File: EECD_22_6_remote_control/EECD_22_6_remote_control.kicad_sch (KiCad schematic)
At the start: 22 parts, among them SW1 SW_SPDT, U1 NRF24L01_Breakout, U2 NUCLEO144-F746ZG

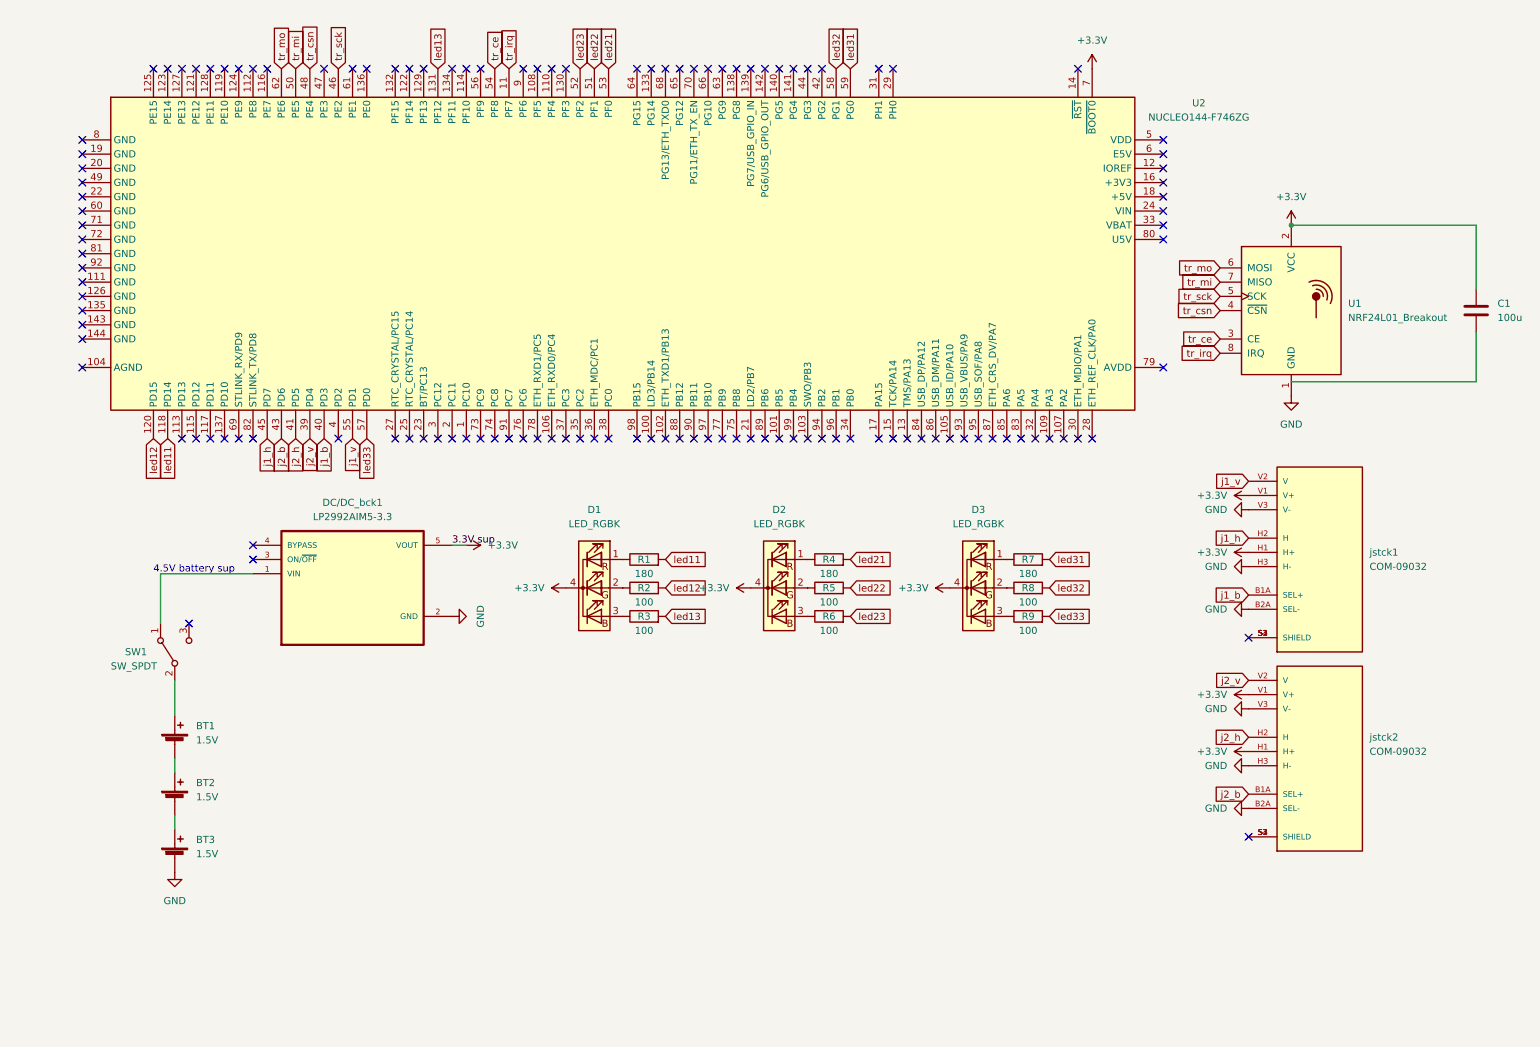
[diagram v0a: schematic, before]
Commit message: you can understand at least smth now
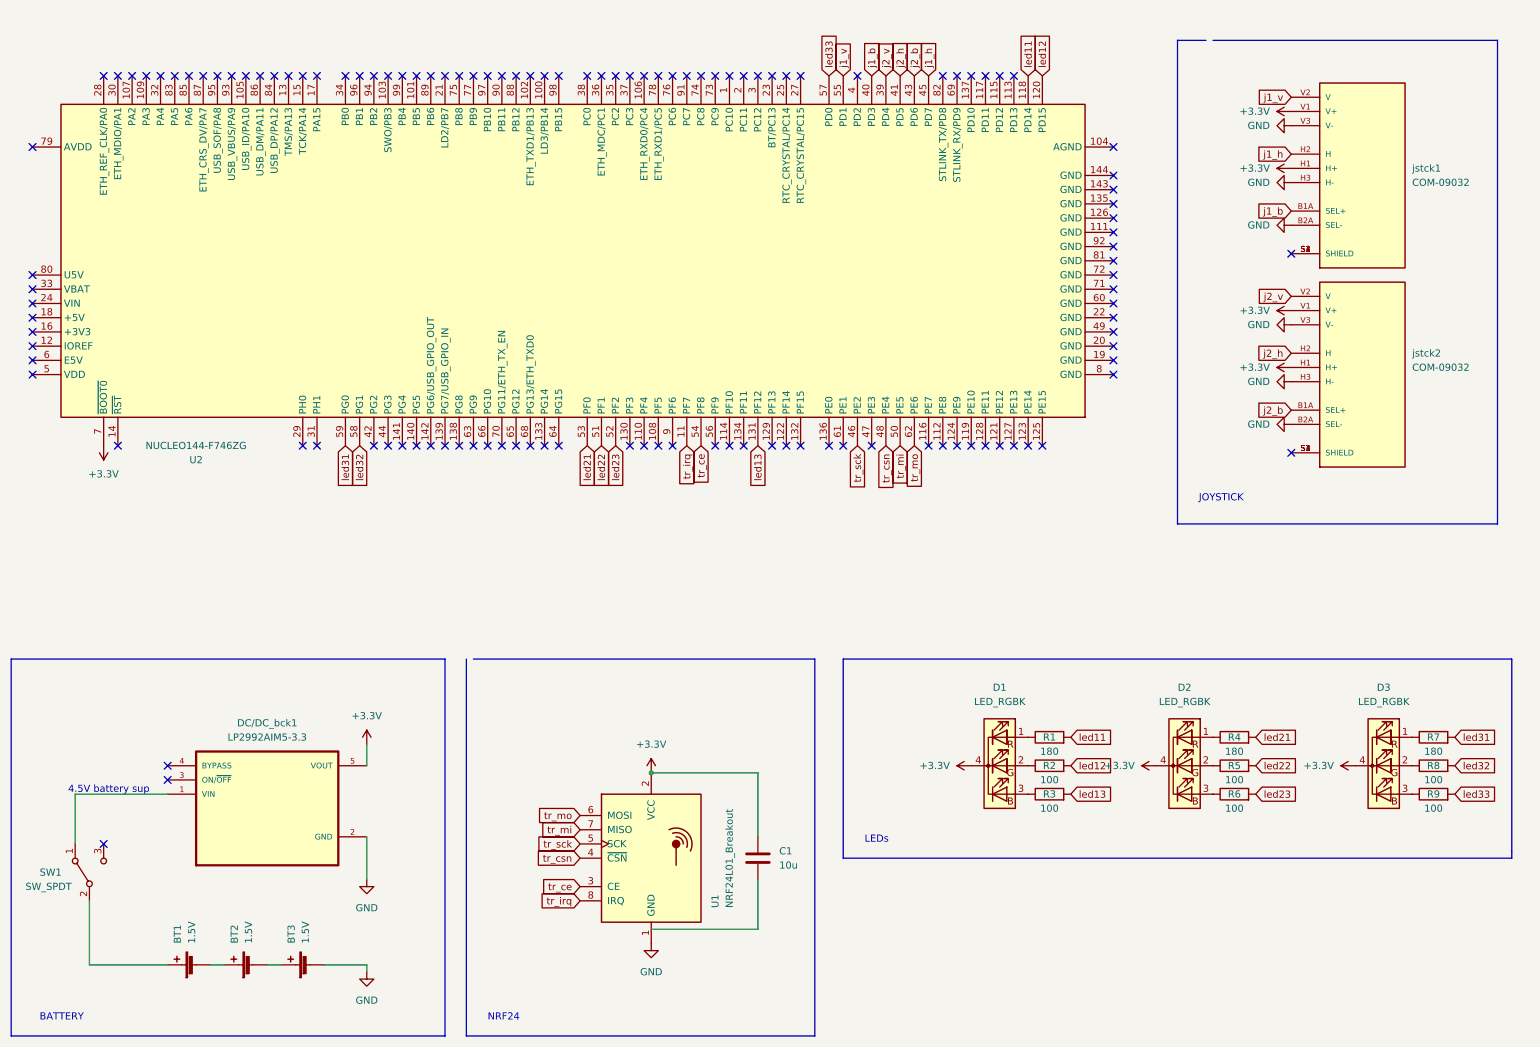
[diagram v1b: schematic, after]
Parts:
- C1: value 100u -> 10u
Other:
- note added: "BATTERY"
- note added: "JOYSTICK"
- note added: "LEDs"
- note added: "NRF24"
- moved on the sheet: BT1, BT2, BT3, C1, D1, D2, D3, DC/DC_bck1, R1, R2, R3, R4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
